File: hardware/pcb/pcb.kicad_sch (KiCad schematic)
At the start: 21 parts, among them J1 Raspberry_Pi_2_3

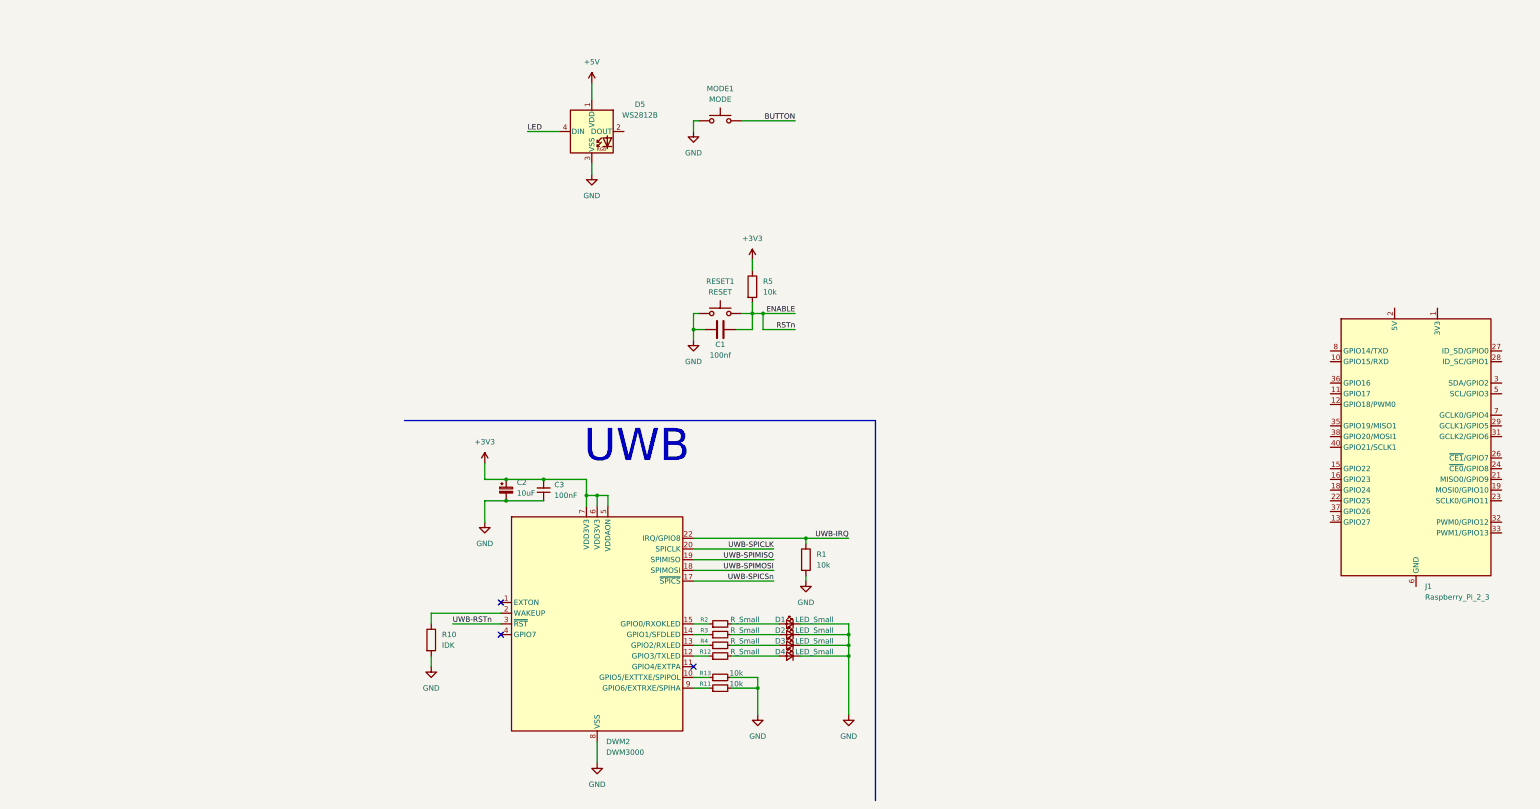
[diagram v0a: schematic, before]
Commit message: Added IMU
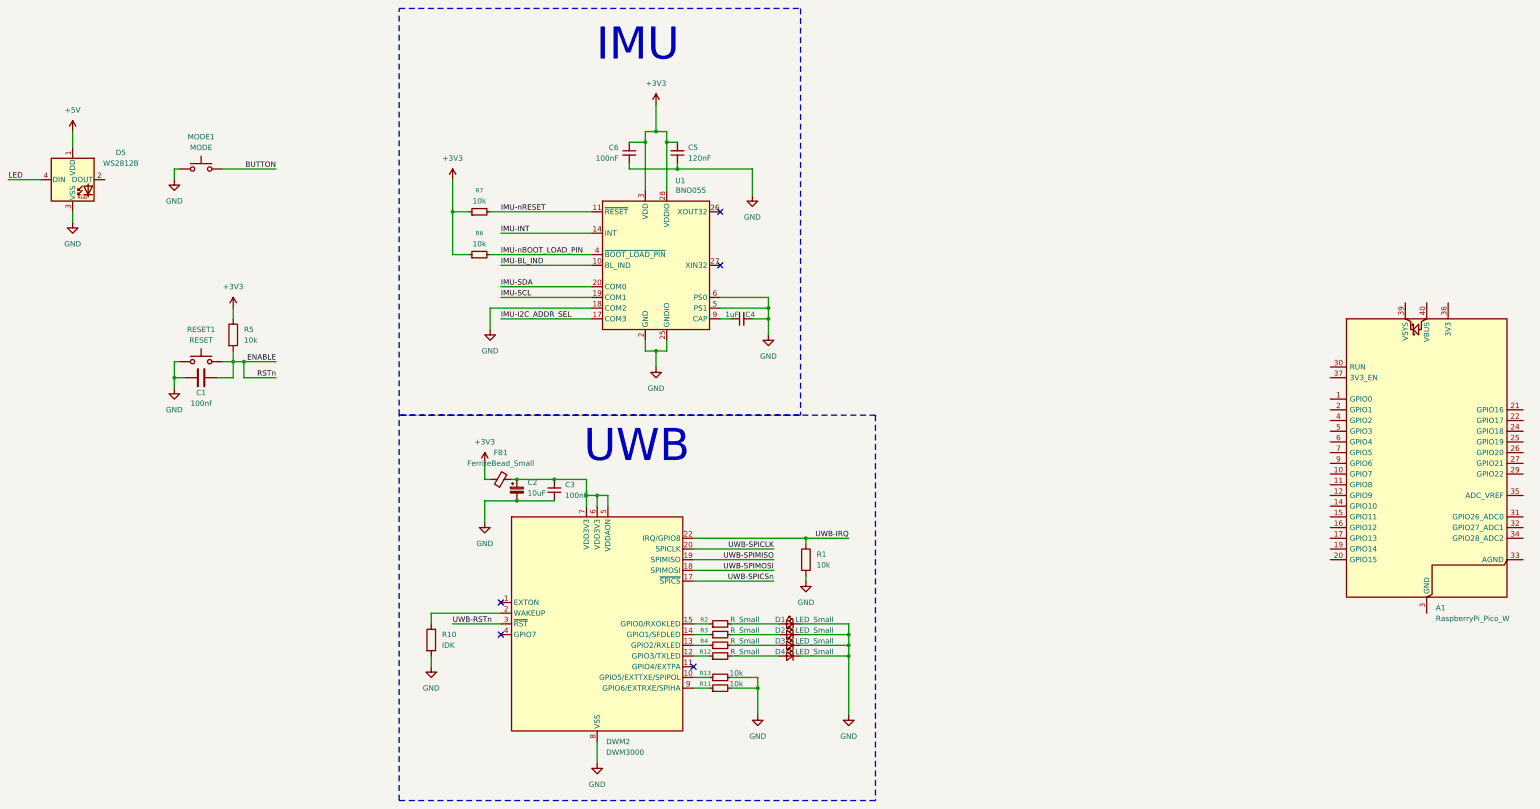
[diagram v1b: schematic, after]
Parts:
- removed J1: Raspberry_Pi_2_3, Module:RaspberryPi_Pico_Common_Unspecified, symbol Connector:Raspberry_Pi_2_3
- added A1: RaspberryPi_Pico_W, Module:RaspberryPi_Pico_Common_Unspecified, symbol MCU_Module:RaspberryPi_Pico_W
- added C4: 1uF, symbol Device:C_Small
- added C5: 120nF, symbol Device:C_Small
- added C6: 100nF, symbol Device:C_Small
- added FB1: FerriteBead_Small, symbol Device:FerriteBead_Small
- added R6, R7: 10k, symbol Device:R_Small
- added U1: BNO055, Package_LGA:LGA-28_5.2x3.8mm_P0.5mm, symbol Sensor_Motion:BNO055
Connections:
- net +3V3: now also C5.2, C6.1, FB1.1, R6.1, R7.1, U1.28 (VDDIO), U1.3 (VDD); no longer C2.1, C3.2, DWM2.5 (VDDAON), DWM2.6 (VDD3V3), DWM2.7 (VDD3V3)
- net GND: now also C4.2, C5.1, C6.2, U1.18 (COM2), U1.2 (GND), U1.25 (GNDIO), U1.5 (PS1), U1.6 (PS0)
- new net: C2.1, C3.2, DWM2.5 (VDDAON), DWM2.6 (VDD3V3), DWM2.7 (VDD3V3), FB1.2
- new net: C4.1, U1.9 (CAP)
- new net: A1.13 (GND), A1.18 (GND), A1.23 (GND), A1.28 (GND), A1.3 (GND), A1.38 (GND), A1.8 (GND)
- new net IMU-BL_IND: U1.10 (BL_IND)
- new net IMU-I2C_ADDR_SEL: U1.17 (COM3)
- new net IMU-INT: U1.14 (INT)
- new net IMU-SCL: U1.19 (COM1)
- new net IMU-SDA: U1.20 (COM0)
- new net IMU-nBOOT_LOAD_PIN: R6.2, U1.4 (~{BOOT_LOAD_PIN})
- new net IMU-nRESET: R7.2, U1.11 (~{RESET})
- no-connect marks 3 -> 5
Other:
- note added: "IMU"
- moved on the sheet: C1, C2, C3, D5, MODE1, R5, RESET1
